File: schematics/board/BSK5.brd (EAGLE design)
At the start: 94 x 94 mm, 89 parts, among them U1 STM32F405RGT6, X1 JST-6, X11 JST-6

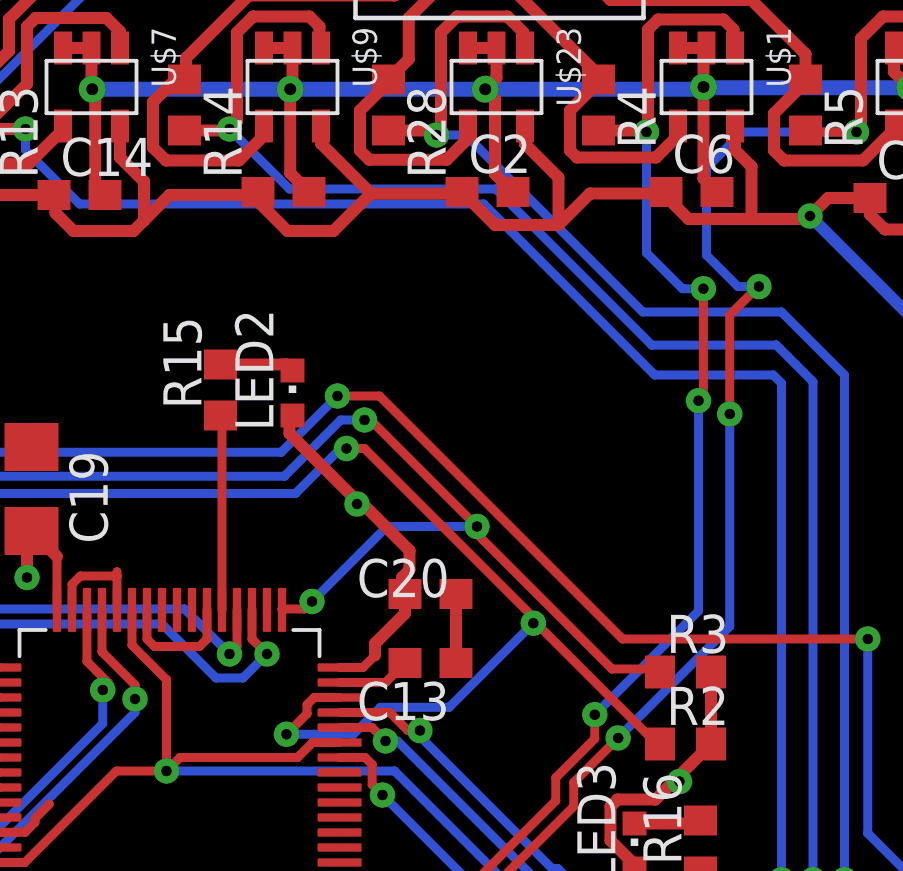
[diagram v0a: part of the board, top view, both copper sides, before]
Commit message: Начато исправление разъемов
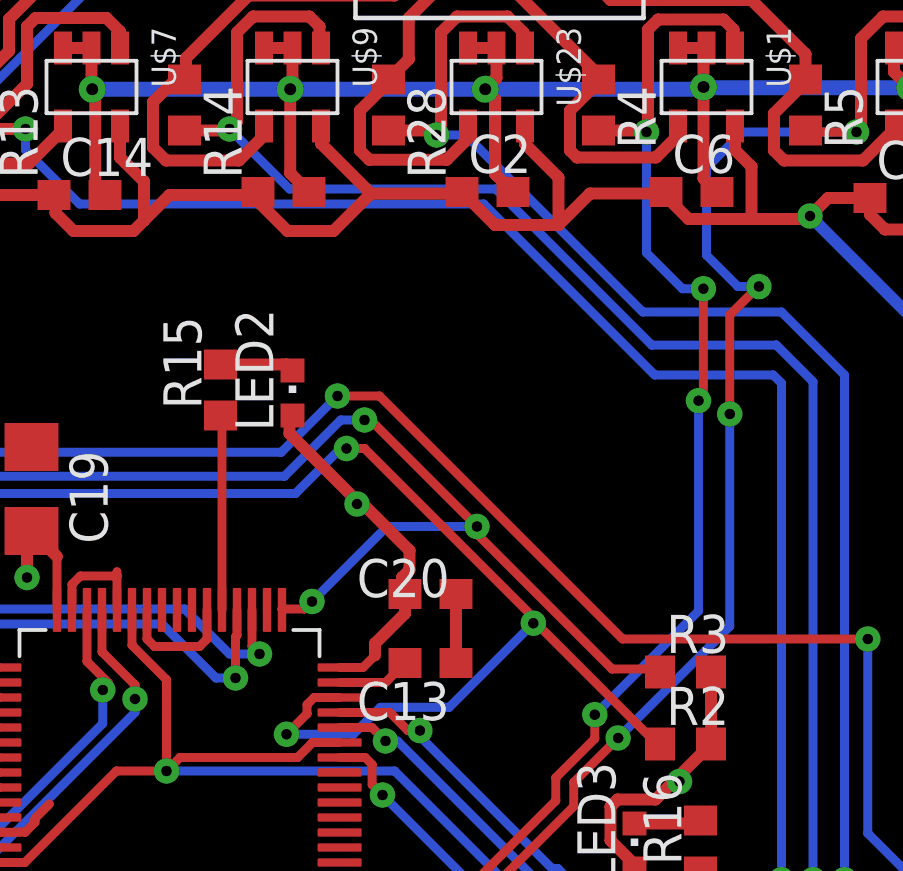
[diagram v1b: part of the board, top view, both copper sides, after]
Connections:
- net RX-S: now also U1.52; no longer U1.51
- net TX-S: now also U1.51; no longer U1.52
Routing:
- net TX-S: track 40.6 -> 41.6 mm
- net RX-S: track 41.5 -> 40.8 mm
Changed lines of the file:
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@@
 <wire x1="58.55" y1="19.8" x2="58.75" y2="19.6" width="0.4" layer="1"/>
 <wire x1="58.85" y1="64.4" x2="59.05" y2="64.2" width="0.4" layer="1"/>
-<wire x1="52.05" y1="64.6" x2="52.25" y2="64.4" width="0.4" layer="1"/>
 <wire x1="45.25" y1="64.6" x2="45.45" y2="64.4" width="0.4" layer="1"/>
 <wire x1="38.45" y1="64.6" x2="38.65" y2="64.4" width="0.4" layer="1"/>
@@
 </signal>
 <signal name="RX-S">
-<contactref element="U1" pad="51"/>
 <wire x1="11.25" y1="55.5" x2="10.75" y2="55.5" width="0.3" layer="16"/>
 <wire x1="16.75" y1="50" x2="11.25" y2="55.5" width="0.3" layer="16"/>
 <wire x1="33.75" y1="50" x2="16.75" y2="50" width="0.3" layer="16"/>
 <wire x1="35.55" y1="48.2" x2="33.75" y2="50" width="0.3" layer="16"/>
-<wire x1="36.45" y1="48.2" x2="35.55" y2="48.2" width="0.3" layer="16"/>
-<wire x1="37.25" y1="49" x2="36.45" y2="48.2" width="0.3" layer="16"/>
-<wire x1="36.75" y1="49.5" x2="37.25" y2="49" width="0.3" layer="1"/>
-<wire x1="36.75" y1="50.47" x2="36.75" y2="49.5" width="0.3" layer="1"/>
+<wire x1="35.55" y1="48.2" x2="36.2" y2="48.2" width="0.3" layer="16"/>
 <via x="10.75" y="55.5" extent="1-16" drill="0.35"/>
-<via x="37.25" y="49" extent="1-16" drill="0.35"/>
 <contactref element="U$12" pad="P$4"/>
 <wire x1="10.75" y1="55.5" x2="10.75" y2="56.45" width="0.3" layer="1"/>
@@
 <via x="3.7" y="57" extent="1-16" drill="0.35"/>
 <wire x1="3.7" y1="57" x2="5.05" y2="57" width="0.3" layer="16"/>
+<contactref element="U1" pad="52"/>
+<via x="36.2" y="48.2" extent="1-16" drill="0.35"/>
+<wire x1="36.2" y1="49.570525" x2="36.2" y2="48.2" width="0.3" layer="1"/>
+<wire x1="36.25" y1="50.47" x2="36.25" y2="49.620525" width="0.3" layer="1"/>
+<wire x1="36.25" y1="49.620525" x2="36.2" y2="49.570525" width="0.3" layer="1"/>
 </signal>
 <signal name="TX-S">
-<contactref element="U1" pad="52"/>
 <wire x1="9.15" y1="60.55" x2="8.75" y2="60.55" width="0.3" layer="16"/>
 <wire x1="19.2" y1="50.5" x2="9.15" y2="60.55" width="0.3" layer="16"/>
 <wire x1="34.5" y1="50.5" x2="19.2" y2="50.5" width="0.3" layer="16"/>
-<wire x1="36" y1="49" x2="34.5" y2="50.5" width="0.3" layer="16"/>
-<wire x1="36.25" y1="49.25" x2="36" y2="49" width="0.3" layer="1"/>
-<wire x1="36.25" y1="50.47" x2="36.25" y2="49.25" width="0.3" layer="1"/>
+<wire x1="34.5" y1="50.5" x2="36" y2="49" width="0.3" layer="16"/>
 <via x="8.75" y="60.55" extent="1-16" drill="0.35"/>
-<via x="36" y="49" extent="1-16" drill="0.35"/>
 <contactref element="U$12" pad="P$6"/>
 <wire x1="8.75" y1="60.55" x2="7.2" y2="59" width="0.3" layer="1"/>
@@
 <via x="3.7" y="59" extent="1-16" drill="0.35"/>
 <wire x1="3.7" y1="59" x2="5.05" y2="59" width="0.3" layer="16"/>
+<contactref element="U1" pad="51"/>
+<wire x1="36" y1="49" x2="37" y2="49" width="0.3" layer="16"/>
+<via x="37" y="49" extent="1-16" drill="0.35"/>
+<wire x1="37" y1="49" x2="36.75" y2="49.25" width="0.3" layer="1"/>
+<wire x1="36.75" y1="49.25" x2="36.75" y2="50.47" width="0.3" layer="1"/>
 </signal>
 <signal name="SWC">
